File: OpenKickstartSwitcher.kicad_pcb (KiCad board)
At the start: 2 copper layers, 25.7 x 79.2 mm, 13 parts, among them J1 Conn_01x03, J2 Conn_01x04, J4 Conn_01x03, J98 LOGO, J99 OSHW_LOGO, U1 KS_SOCKET, U2 M27C800, U3 7400

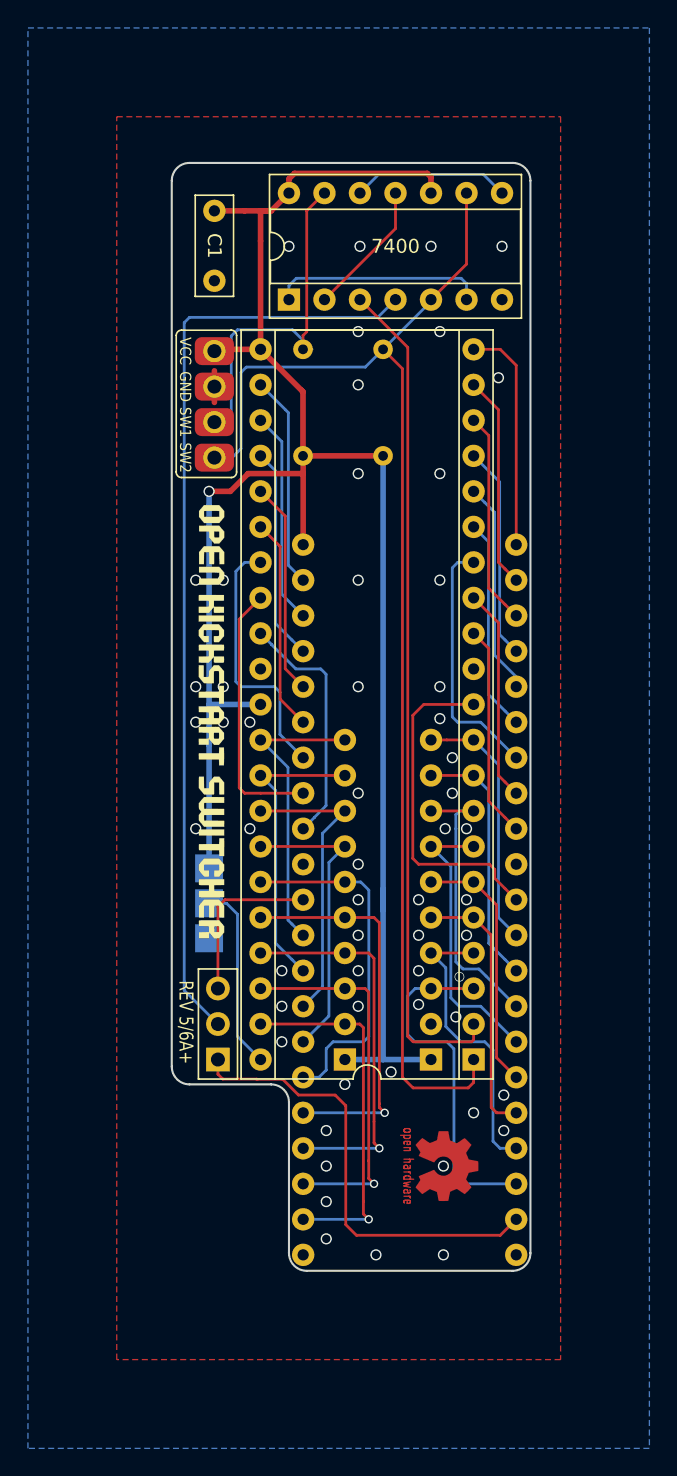
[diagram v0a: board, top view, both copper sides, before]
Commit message: Ready for V1-cdtv!
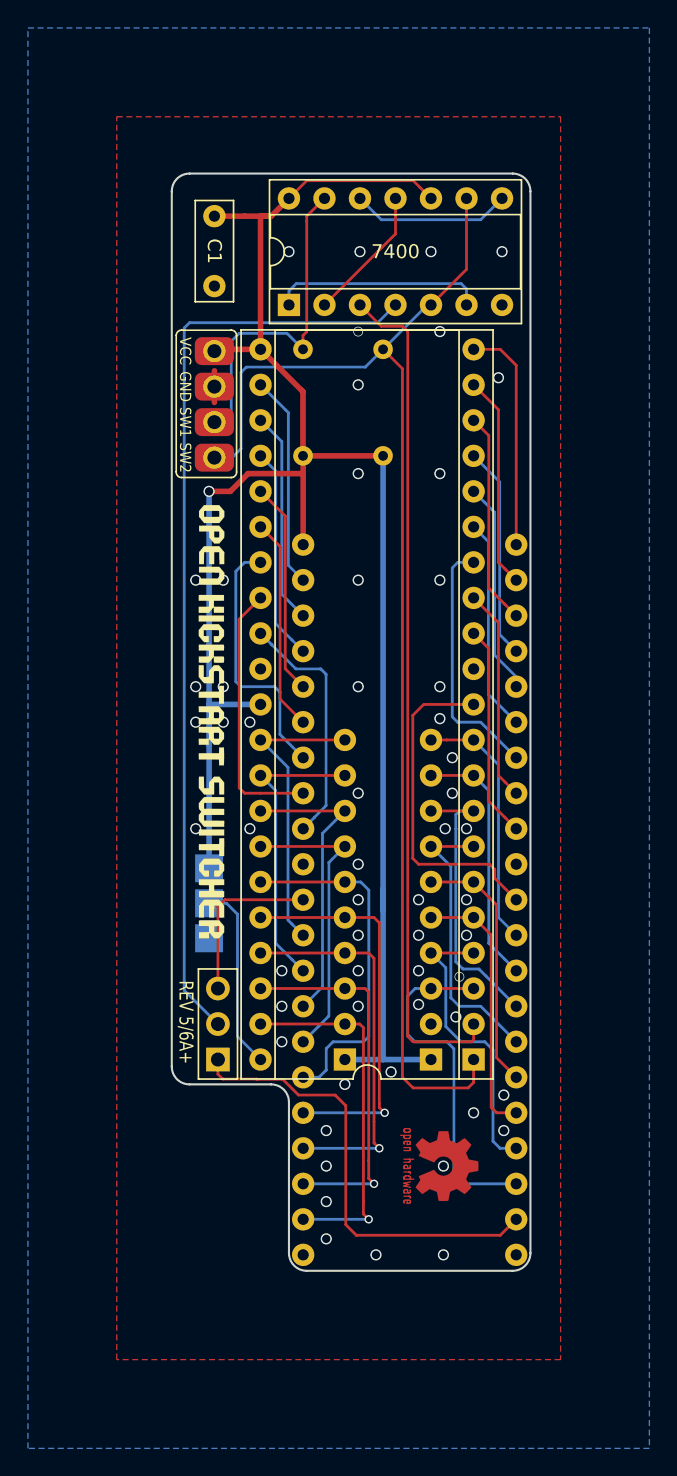
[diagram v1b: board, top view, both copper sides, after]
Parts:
- moved C1 0.38 mm to (146.7, 89.7)
- moved U3 0.38 mm to (152.0, 96.0)
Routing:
- net VCC: track 142.6 -> 140.9 mm
- net /sw17: track 25.6 -> 24.1 mm
- net Net-(U2-Pad2): track 60.2 -> 60.7 mm
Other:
- board size 25.7 x 79.2 mm -> 25.7 x 78.5 mm
